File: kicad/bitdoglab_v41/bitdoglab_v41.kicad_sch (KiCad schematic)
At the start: 45 parts, among them J1 Conn_01x20_Socket, J10 GND, J11 GND, J12 Conn_01x05_Pin, J13 Conn_01x05_Pin, J14 5x5 Matrix led, J15 GND, J16 GND, J17 GND, J18 GND, J19 JOYSTICK, J2 conector_idc, J3 Conn_01x20_Socket, J4 jumper_mic, J5 Conn_01x05_Pin, J6 Conn_01x05_Pin, J7 GND, J8 GND, J9 GND, Q1 DMG2305UX-13, Q2 BC337, Q3 BC337, SW1 RESET, SW2 Button_A, SW3 Button_B, U1 3.3v_tht, U2 3.3v_smd, U3 BAT (DIS)CHARGE, U4 1063

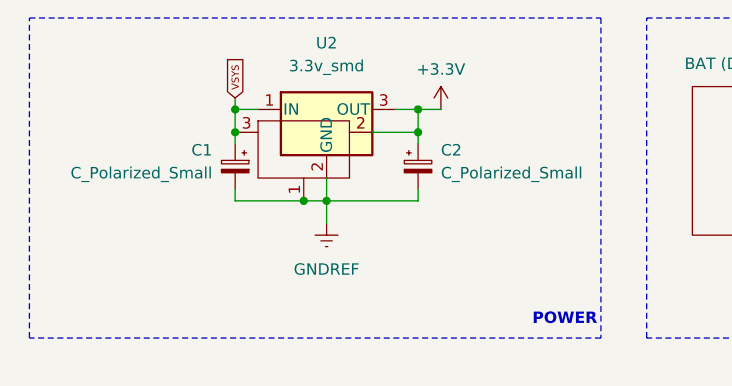
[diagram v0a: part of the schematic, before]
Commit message: versao 4.1 diretamente no layout
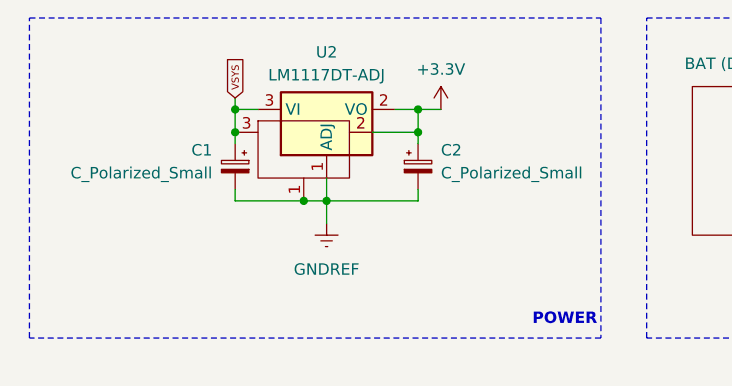
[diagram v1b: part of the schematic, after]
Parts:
- removed U2: 3.3v_smd, Package_TO_SOT_SMD:SOT-223, symbol Regulator_Linear:uA7805
- added U2: LM1117DT-ADJ, Package_TO_SOT_SMD:TO-252-3_TabPin2, symbol Regulator_Linear:LM1117DT-ADJ
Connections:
- net +3.3V: now also U2.2 (VO)
- net GNDREF: now also U2.1 (ADJ)
- net VSYS: now also U2.3 (VI)
